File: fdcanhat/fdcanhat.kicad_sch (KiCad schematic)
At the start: 2 parts, among them J1 Raspberry_Pi_5, J2 GH1.25-8P

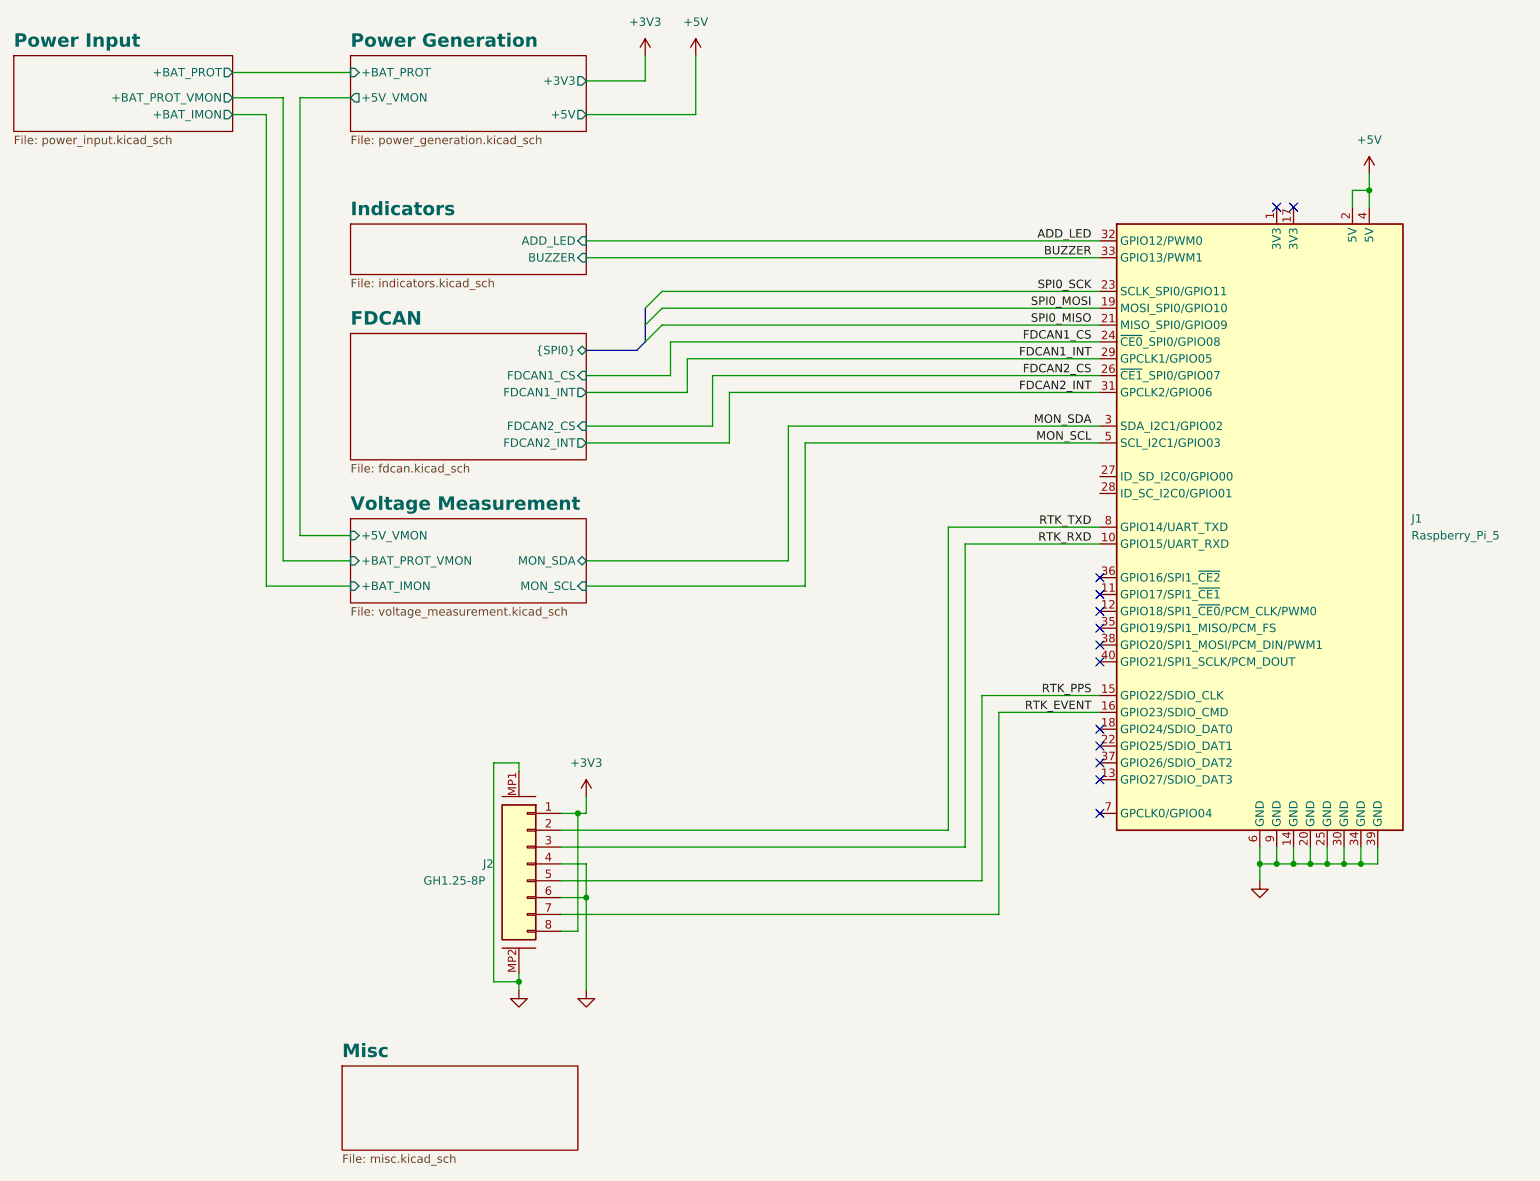
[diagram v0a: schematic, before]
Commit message: almost done
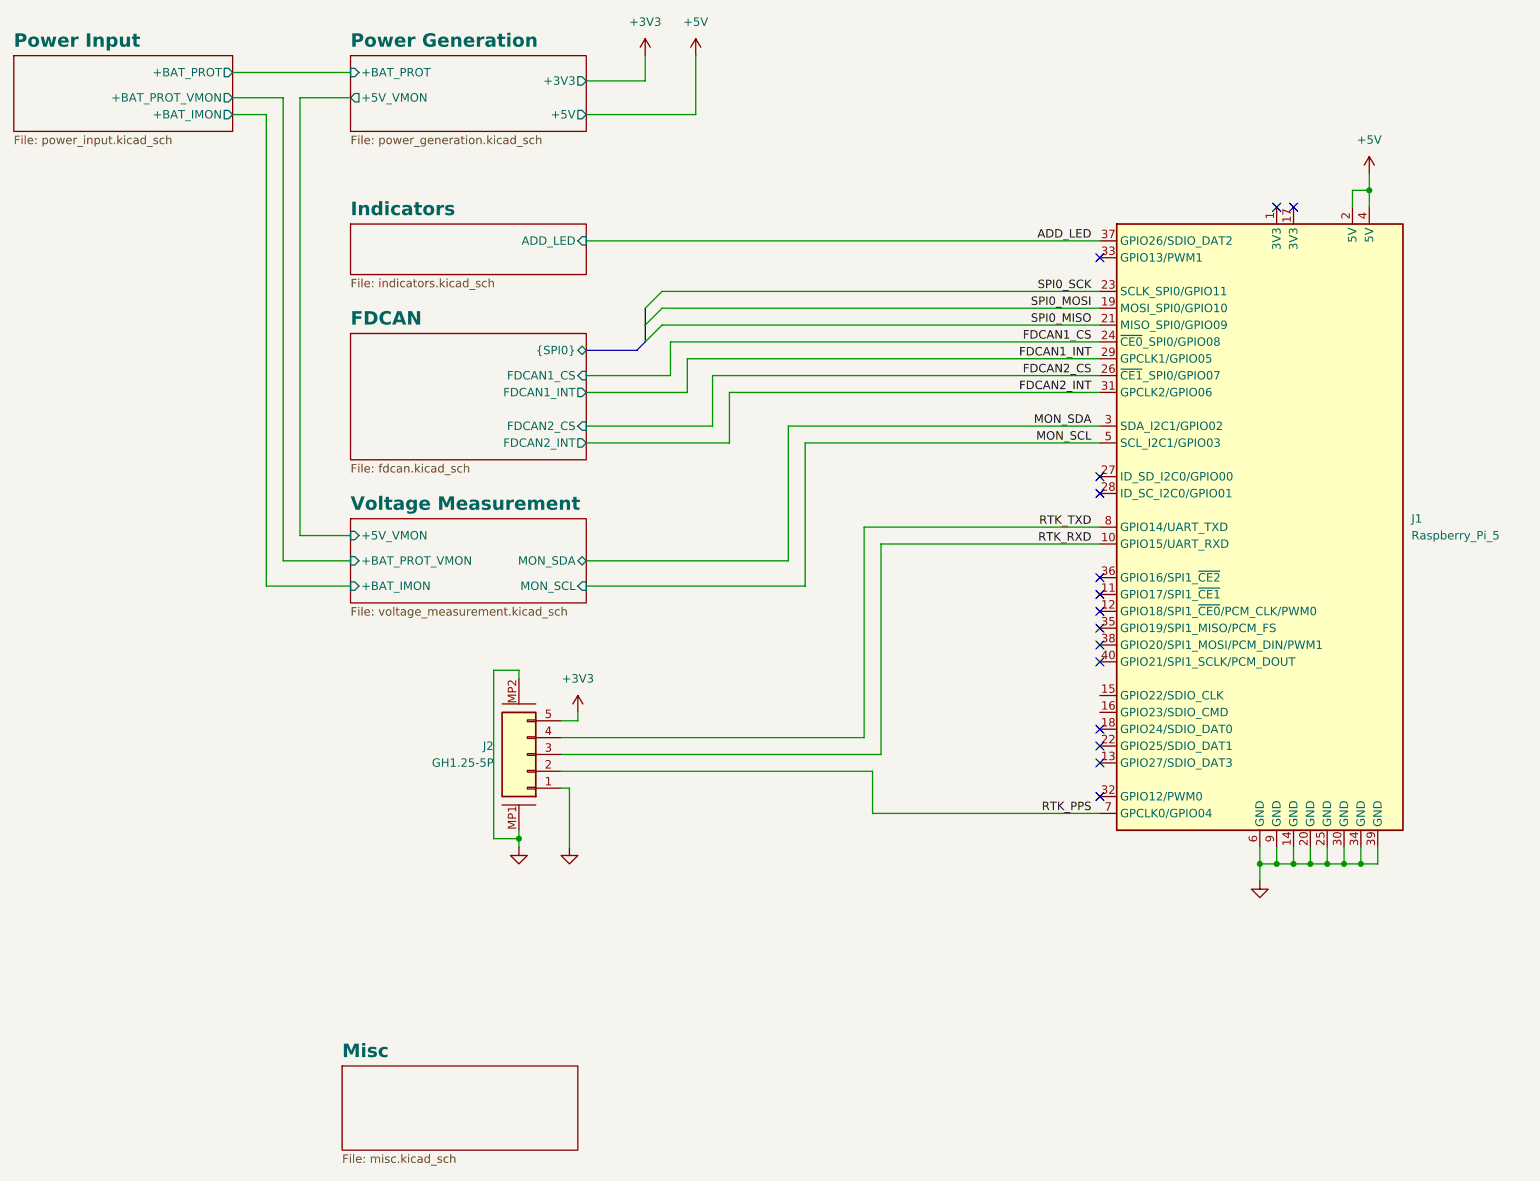
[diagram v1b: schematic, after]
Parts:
- removed J2: GH1.25-8P, 0_connectors:SM08B-GHS-TB-LF-SN, symbol 0_connectors:Conn_01x08_Mounting
- added J2: GH1.25-5P, 0_connectors:SM05B-GHS-TB-LF-SN, symbol 0_connectors:Conn_01x05_Mounting
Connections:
- net +3V3: now also J2.5 (Pin_5)
- net ADD_LED: now also J1.37 (GPIO26/SDIO_DAT2); no longer J1.32 (GPIO12/PWM0)
- net GND: now also J2.1 (Pin_1), J2.MP1, J2.MP2
- net RTK_PPS: now also J1.7 (GPCLK0/GPIO04), J2.2 (Pin_2); no longer J1.15 (GPIO22/SDIO_CLK)
- net RTK_RXD: now also J2.3 (Pin_3)
- net RTK_TXD: now also J2.4 (Pin_4)
- net BUZZER: no longer names the net of J1.33 (GPIO13/PWM1)
- net RTK_EVENT: no longer names the net of J1.16 (GPIO23/SDIO_CMD)
- no-connect marks 13 -> 15
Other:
- sheet Indicators ports: added none; removed BUZZER
